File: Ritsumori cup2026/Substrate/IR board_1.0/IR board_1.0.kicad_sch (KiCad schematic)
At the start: 32 parts, among them IC1 STM32F446RET6, J1 PC, J2 main, SW1 SW_Push, SW2 SW_Push, U1 TSSP4038, U10 TSSP4038, U11 TSSP4038, U12 TSSP4038, U13 TSSP4038, U14 TSSP4038, U15 TSSP4038, U16 TSSP4038, U2 TSSP4038, U3 TSSP4038, U4 TSSP4038, U5 TSSP4038, U6 TSSP4038, U7 TSSP4038, U8 TSSP4038, U9 TSSP4038

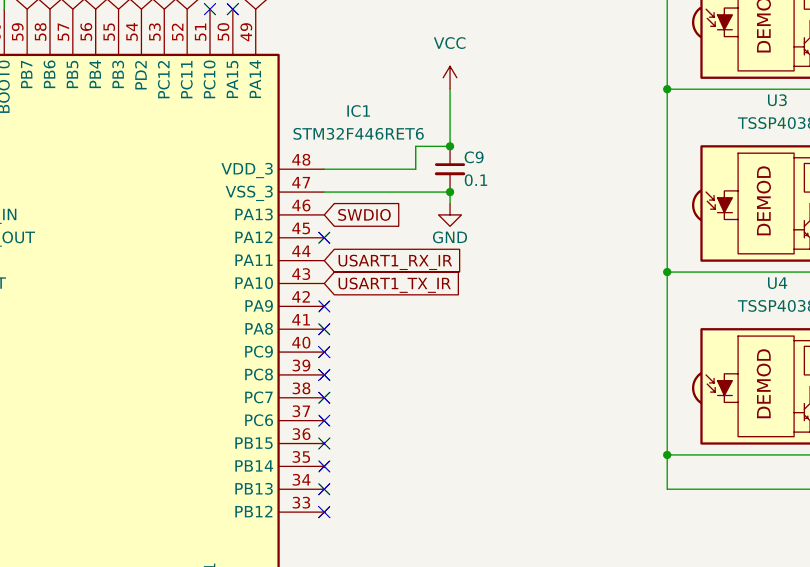
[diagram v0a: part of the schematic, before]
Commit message: Auto Backup: 2026/03/09 13:07:55.49
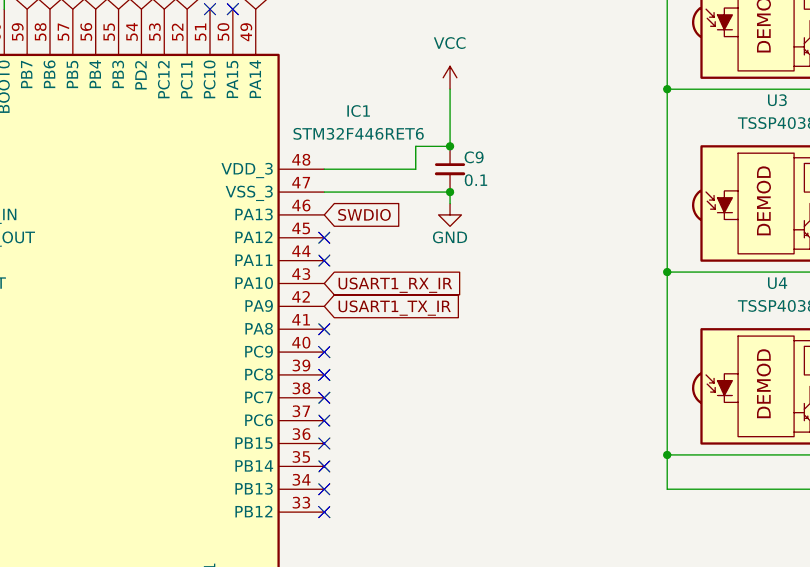
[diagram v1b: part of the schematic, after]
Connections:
- net USART1_RX_IR: now also IC1.43 (PA10); no longer IC1.44 (PA11)
- net USART1_TX_IR: now also IC1.42 (PA9); no longer IC1.43 (PA10)
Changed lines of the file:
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@@
+	)
+	(no_connect
+		(at 95.25 81.28)
 	)
 	(no_connect
@@
 	)
 	(no_connect
-		(at 95.25 86.36)
-	)
-	(no_connect
 		(at 77.47 127)
 	)
@@
 	(global_label "USART1_RX_IR"
 		(shape input)
-		(at 95.25 81.28 0)
+		(at 95.25 83.82 0)
 		(fields_autoplaced yes)
 		(effects
@@
 		)
 		(property "Intersheetrefs" "${INTERSHEET_REFS}"
-			(at 111.6004 81.28 0)
+			(at 111.6004 83.82 0)
 			(effects
 				(font
@@
 	(global_label "USART1_TX_IR"
 		(shape input)
-		(at 95.25 83.82 0)
+		(at 95.25 86.36 0)
 		(fields_autoplaced yes)
 		(effects
@@
 		)
 		(property "Intersheetrefs" "${INTERSHEET_REFS}"
-			(at 111.298 83.82 0)
-			(effects
-				(font
+			(at 111.298 86.36 0)
+			(effects
+				(font
